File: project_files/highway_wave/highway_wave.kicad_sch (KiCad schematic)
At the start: 12 parts, among them U1 ESP32-S3, U4 PAM8403D

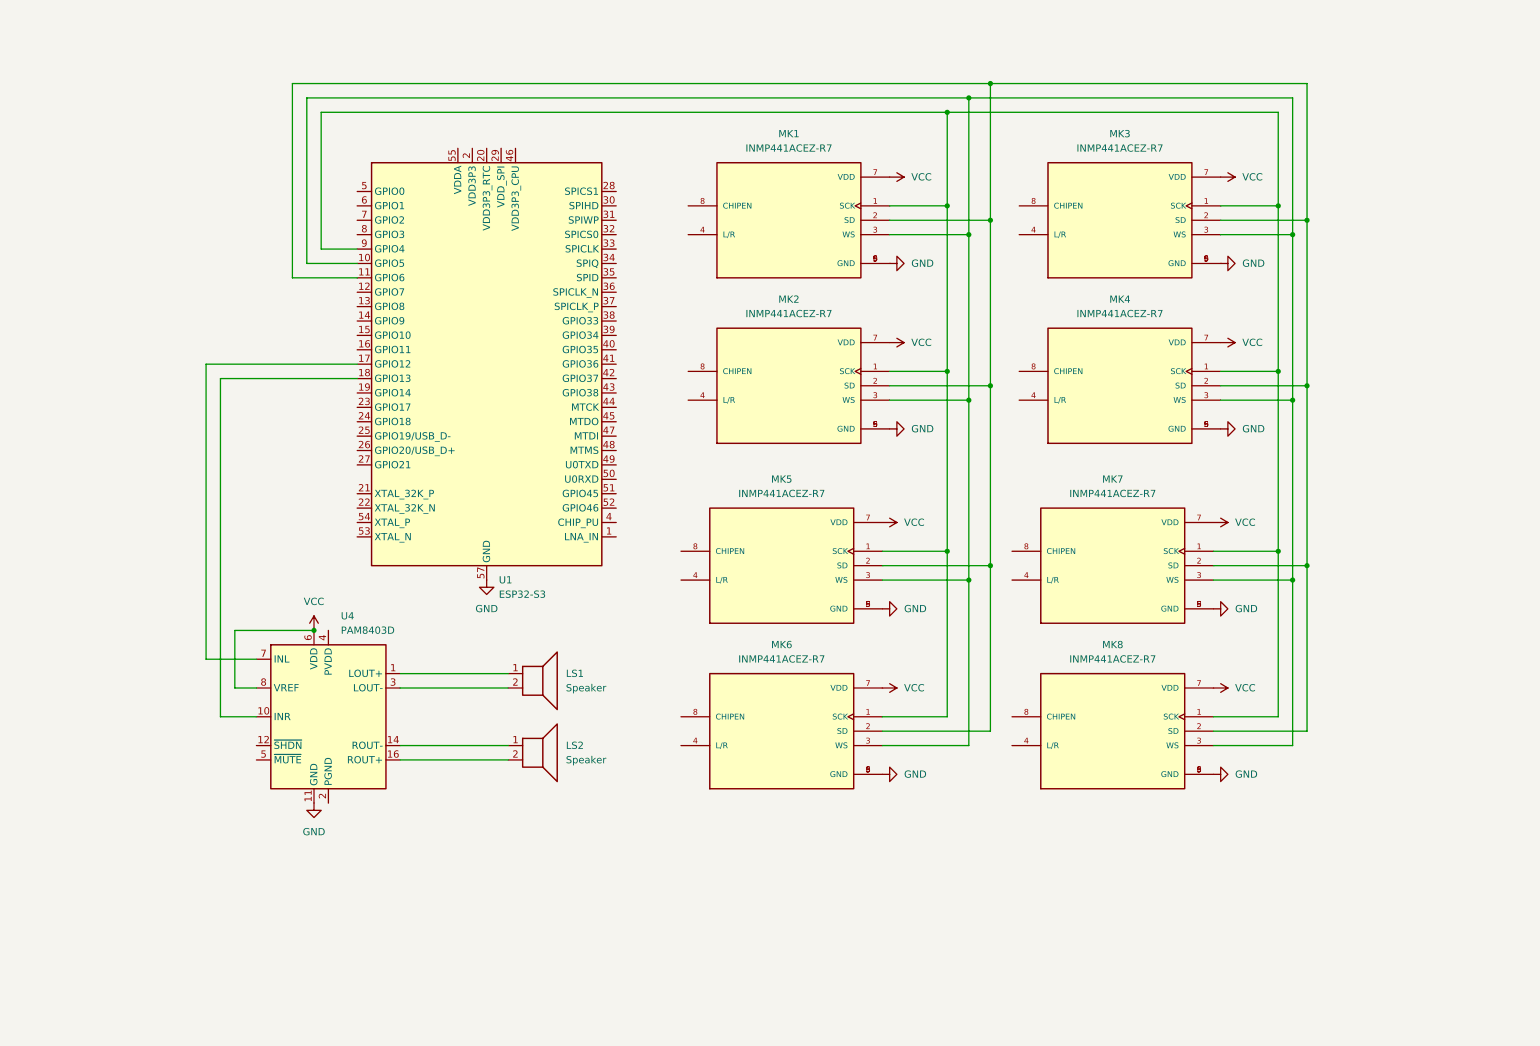
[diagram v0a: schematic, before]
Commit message: big updates to pcb
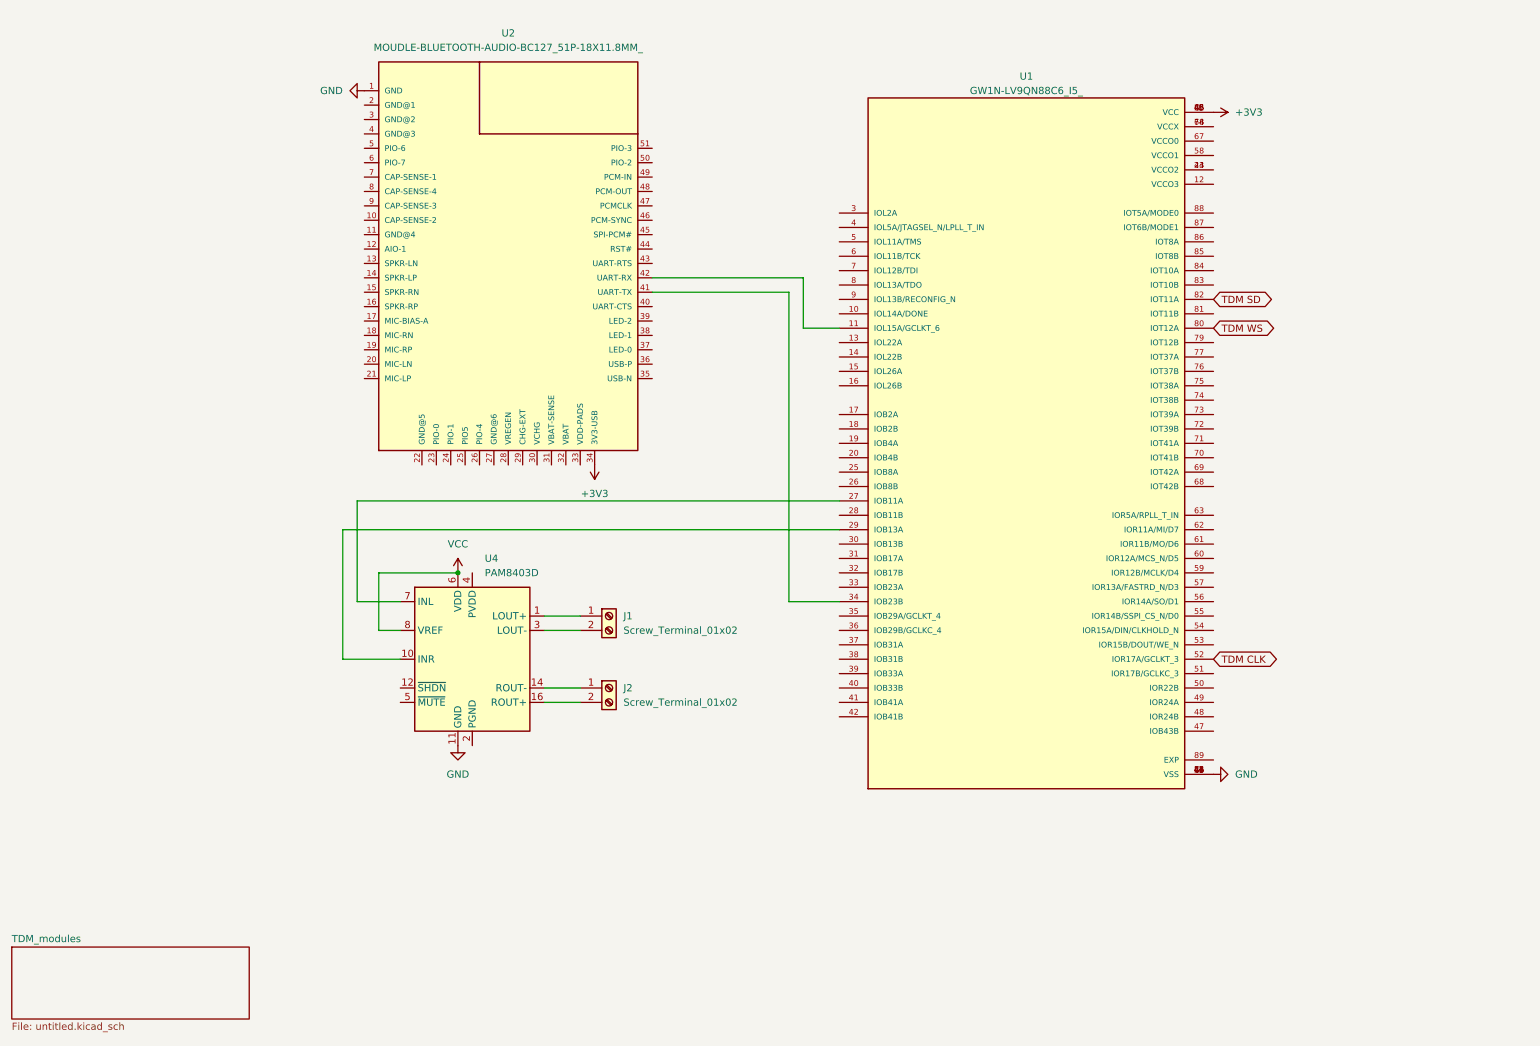
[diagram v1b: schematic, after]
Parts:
- removed LS1, LS2: Speaker, symbol Device:Speaker
- removed MK1, MK2, MK3, MK4, MK5, MK6, MK7, MK8: INMP441ACEZ-R7, INMP441ACEZ-R7:MIC_INMP441ACEZ-R7, symbol INMP441ACEZ-R7:INMP441ACEZ-R7
- removed U1: ESP32-S3, Package_DFN_QFN:QFN-56-1EP_7x7mm_P0.4mm_EP4x4mm, symbol MCU_Espressif:ESP32-S3
- added J1, J2: Screw_Terminal_01x02, TerminalBlock_MetzConnect:TerminalBlock_MetzConnect_Type101_RT01602HBWC_1x02_P5.08mm_Horizontal, symbol Connector:Screw_Terminal_01x02
- added U1: GW1N-LV9QN88C6_I5_, GW1N-LV9QN88C6_I5_:QFN40P1000X1000X95-89N, symbol GW1N-LV9QN88C6_I5_:GW1N-LV9QN88C6_I5_
- added U2: MOUDLE-BLUETOOTH-AUDIO-BC127_51P-18X11.8MM_, MOUDLE-BLUETOOTH-AUDIO-BC127_51P-18X11.8MM_:LGA51-0.8-18X11.8MM, symbol MOUDLE-BLUETOOTH-AUDIO-BC127_51P-18X11.8MM_:MOUDLE-BLUETOOTH-AUDIO-BC127_51P-18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
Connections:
- net GND: now also U1.2 (VSS), U1.21 (VSS), U1.24 (VSS), U1.43 (VSS), U1.46 (VSS), U1.65 (VSS), U2.1 (GND)
- net at U4.7 (INL): now also U1.27 (IOB11A)
- net at U4.10 (INR): now also U1.29 (IOB13A)
- net at U4.14 (ROUT-): now also J2.1 (Pin_1)
- net at U4.16 (ROUT+): now also J2.2 (Pin_2)
- net at U4.1 (LOUT+): now also J1.1 (Pin_1)
- net at U4.3 (LOUT-): now also J1.2 (Pin_2)
- new net: U1.34 (IOB23B), U2.41 (UART-TX)
- new net: U1.11 (IOL15A/GCLKT_6), U2.42 (UART-RX)
- new net: U1.23 (VCCO2), U1.44 (VCCO2)
- new net: U1.64 (VCCX), U1.78 (VCCX)
- new net +3V3: U1.1 (VCC), U1.22 (VCC), U1.45 (VCC), U1.66 (VCC), U2.34 (3V3-USB)
- new net TDM CLK: U1.52 (IOR17A/GCLKT_3)
- new net TDM SD: U1.82 (IOT11A)
- new net TDM WS: U1.80 (IOT12A)
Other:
- added sheet TDM_modules (untitled.kicad_sch)
- moved on the sheet: U4

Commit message: random committ
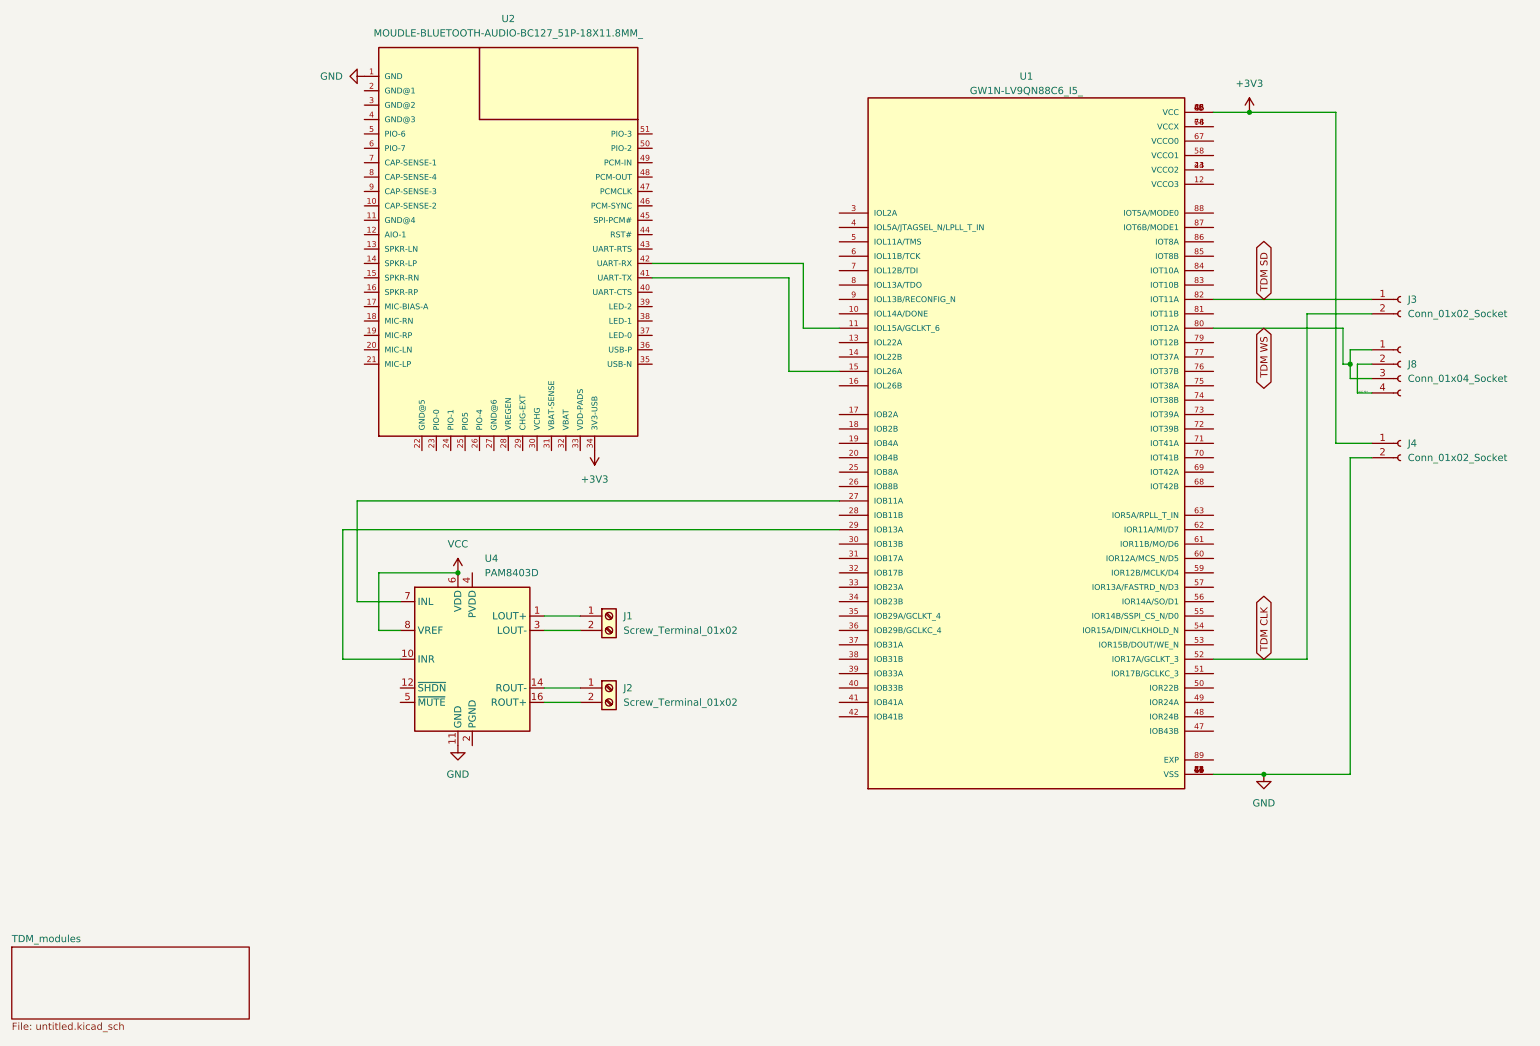
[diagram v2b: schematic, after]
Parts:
- added J3, J4: Conn_01x02_Socket, Connector_Phoenix_GMSTB:PhoenixContact_GMSTBVA_2,5_2-G_1x02_P7.50mm_Vertical, symbol Connector:Conn_01x02_Socket
- added J8: Conn_01x04_Socket, Connector_Phoenix_GMSTB:PhoenixContact_GMSTBVA_2,5_4-G_1x04_P7.50mm_Vertical, symbol Connector:Conn_01x04_Socket
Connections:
- net +3V3: now also J4.1 (Pin_1)
- net GND: now also J4.2 (Pin_2)
- net TDM CLK: now also J3.2 (Pin_2)
- net TDM SD: now also J3.1 (Pin_1)
- net TDM WS: now also J8.1 (Pin_1), J8.3 (Pin_3)
- net at U2.41 (UART-TX): now also U1.15 (IOL26A); no longer U1.34 (IOB23B)
- new net: J8.2 (Pin_2), J8.4 (Pin_4)
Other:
- note added: "WSO Mk4"
- moved on the sheet: U2

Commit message: fixed pcb
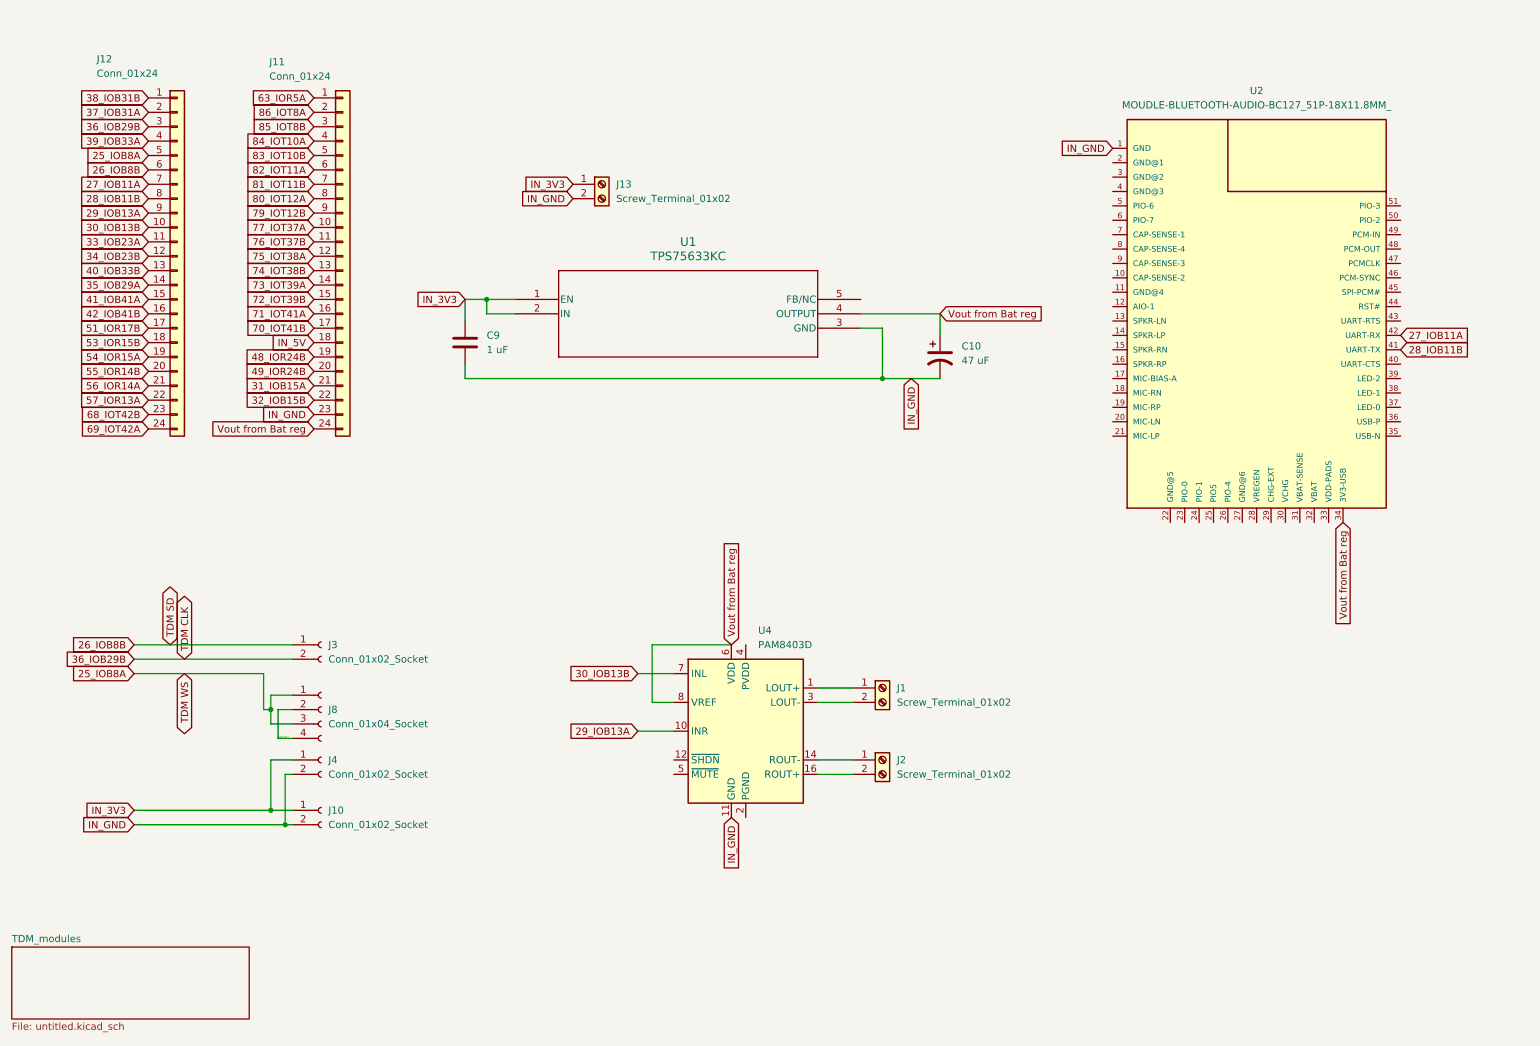
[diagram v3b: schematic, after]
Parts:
- removed U1: GW1N-LV9QN88C6_I5_, GW1N-LV9QN88C6_I5_:QFN40P1000X1000X95-89N, symbol GW1N-LV9QN88C6_I5_:GW1N-LV9QN88C6_I5_
- added C10: 47 uF, Capacitor_THT:CP_Radial_D5.0mm_P2.50mm, symbol Device:C_Polarized_US
- added C9: 1 uF, Capacitor_THT:CP_Radial_D5.0mm_P2.50mm, symbol Device:C
- added J10: Conn_01x02_Socket, Connector_JST:JST_PH_B2B-PH-K_1x02_P2.00mm_Vertical, symbol Connector:Conn_01x02_Socket
- added J11, J12: Conn_01x24, Connector_PinSocket_2.54mm:PinSocket_1x24_P2.54mm_Vertical, symbol Connector_Generic:Conn_01x24
- added J13: Screw_Terminal_01x02, TerminalBlock_MetzConnect:TerminalBlock_MetzConnect_Type101_RT01602HBWC_1x02_P5.08mm_Horizontal, symbol Connector:Screw_Terminal_01x02
- added U1: TPS75633KC, footprints:KC5, symbol Battery Regulator:TPS75633KC
- J3, J4: footprint Connector_Phoenix_GMSTB:PhoenixContact_GMSTBVA_2,5_2-G_1x02_P7.50mm_Vertical -> Connector_JST:JST_PH_B2B-PH-K_1x02_P2.00mm_Vertical
- J8: footprint Connector_Phoenix_GMSTB:PhoenixContact_GMSTBVA_2,5_4-G_1x04_P7.50mm_Vertical -> Connector_JST:JST_PH_B2B-PH-K_1x02_P2.00mm_Vertical
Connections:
- net 28_IOB11B: now reaches U2.41 (UART-TX)
- net 28_IOB11B: now also J12.8 (Pin_8)
- net 27_IOB11A: now reaches U2.42 (UART-RX)
- net 27_IOB11A: now also J12.7 (Pin_7)
- net 30_IOB13B: now reaches U4.7 (INL)
- net 30_IOB13B: now also J12.10 (Pin_10)
- net 29_IOB13A: now reaches U4.10 (INR)
- net 29_IOB13A: now also J12.9 (Pin_9)
- net +3V3 renamed IN_3V3
- net IN_3V3: now also C9.2, J10.1 (Pin_1), J13.1 (Pin_1), U1.1 (EN), U1.2 (IN); no longer U2.34 (3V3-USB)
- net GND renamed IN_GND
- net IN_GND: now also C10.2, C9.1, J10.2 (Pin_2), J11.23 (Pin_23), J13.2 (Pin_2), U1.3 (GND)
- net TDM CLK renamed 36_IOB29B
- net 36_IOB29B: now also J12.3 (Pin_3)
- net TDM SD renamed 26_IOB8B
- net 26_IOB8B: now also J12.6 (Pin_6)
- net TDM WS renamed 25_IOB8A
- net 25_IOB8A: now also J12.5 (Pin_5)
- net VCC renamed Vout from Bat reg
- net Vout from Bat reg: now also U2.34 (3V3-USB), C10.1, J11.24 (Pin_24), U1.4 (OUTPUT)
- new net 31_IOB15A: J11.21 (Pin_21)
- new net 32_IOB15B: J11.22 (Pin_22)
- new net 33_IOB23A: J12.11 (Pin_11)
- new net 34_IOB23B: J12.12 (Pin_12)
- new net 35_IOB29A: J12.14 (Pin_14)
- new net 37_IOB31A: J12.2 (Pin_2)
- new net 38_IOB31B: J12.1 (Pin_1)
- new net 39_IOB33A: J12.4 (Pin_4)
- new net 40_IOB33B: J12.13 (Pin_13)
- new net 41_IOB41A: J12.15 (Pin_15)
- new net 42_IOB41B: J12.16 (Pin_16)
- new net 48_IOR24B: J11.19 (Pin_19)
- new net 49_IOR24B: J11.20 (Pin_20)
- new net 51_IOR17B: J12.17 (Pin_17)
- new net 53_IOR15B: J12.18 (Pin_18)
- new net 54_IOR15A: J12.19 (Pin_19)
- new net 55_IOR14B: J12.20 (Pin_20)
- new net 56_IOR14A: J12.21 (Pin_21)
- new net 57_IOR13A: J12.22 (Pin_22)
- new net 63_IOR5A: J11.1 (Pin_1)
- new net 68_IOT42B: J12.23 (Pin_23)
- new net 69_IOT42A: J12.24 (Pin_24)
- new net 70_IOT41B: J11.17 (Pin_17)
- new net 71_IOT41A: J11.16 (Pin_16)
- new net 72_IOT39B: J11.15 (Pin_15)
- new net 73_IOT39A: J11.14 (Pin_14)
- new net 74_IOT38B: J11.13 (Pin_13)
- new net 75_IOT38A: J11.12 (Pin_12)
- new net 76_IOT37B: J11.11 (Pin_11)
- new net 77_IOT37A: J11.10 (Pin_10)
- new net 79_IOT12B: J11.9 (Pin_9)
- new net 80_IOT12A: J11.8 (Pin_8)
- new net 81_IOT11B: J11.7 (Pin_7)
- new net 82_IOT11A: J11.6 (Pin_6)
- new net 83_IOT10B: J11.5 (Pin_5)
- new net 84_IOT10A: J11.4 (Pin_4)
- new net 85_IOT8B: J11.3 (Pin_3)
- new net 86_IOT8A: J11.2 (Pin_2)
- new net IN_5V: J11.18 (Pin_18)
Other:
- moved on the sheet: J1, J2, J3, J4, J8, U2, U4
